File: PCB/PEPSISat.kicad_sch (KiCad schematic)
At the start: 3 parts, among them U1 STM32H747IITx, U2 RP2350A, U3 MT48LC16M16A2P

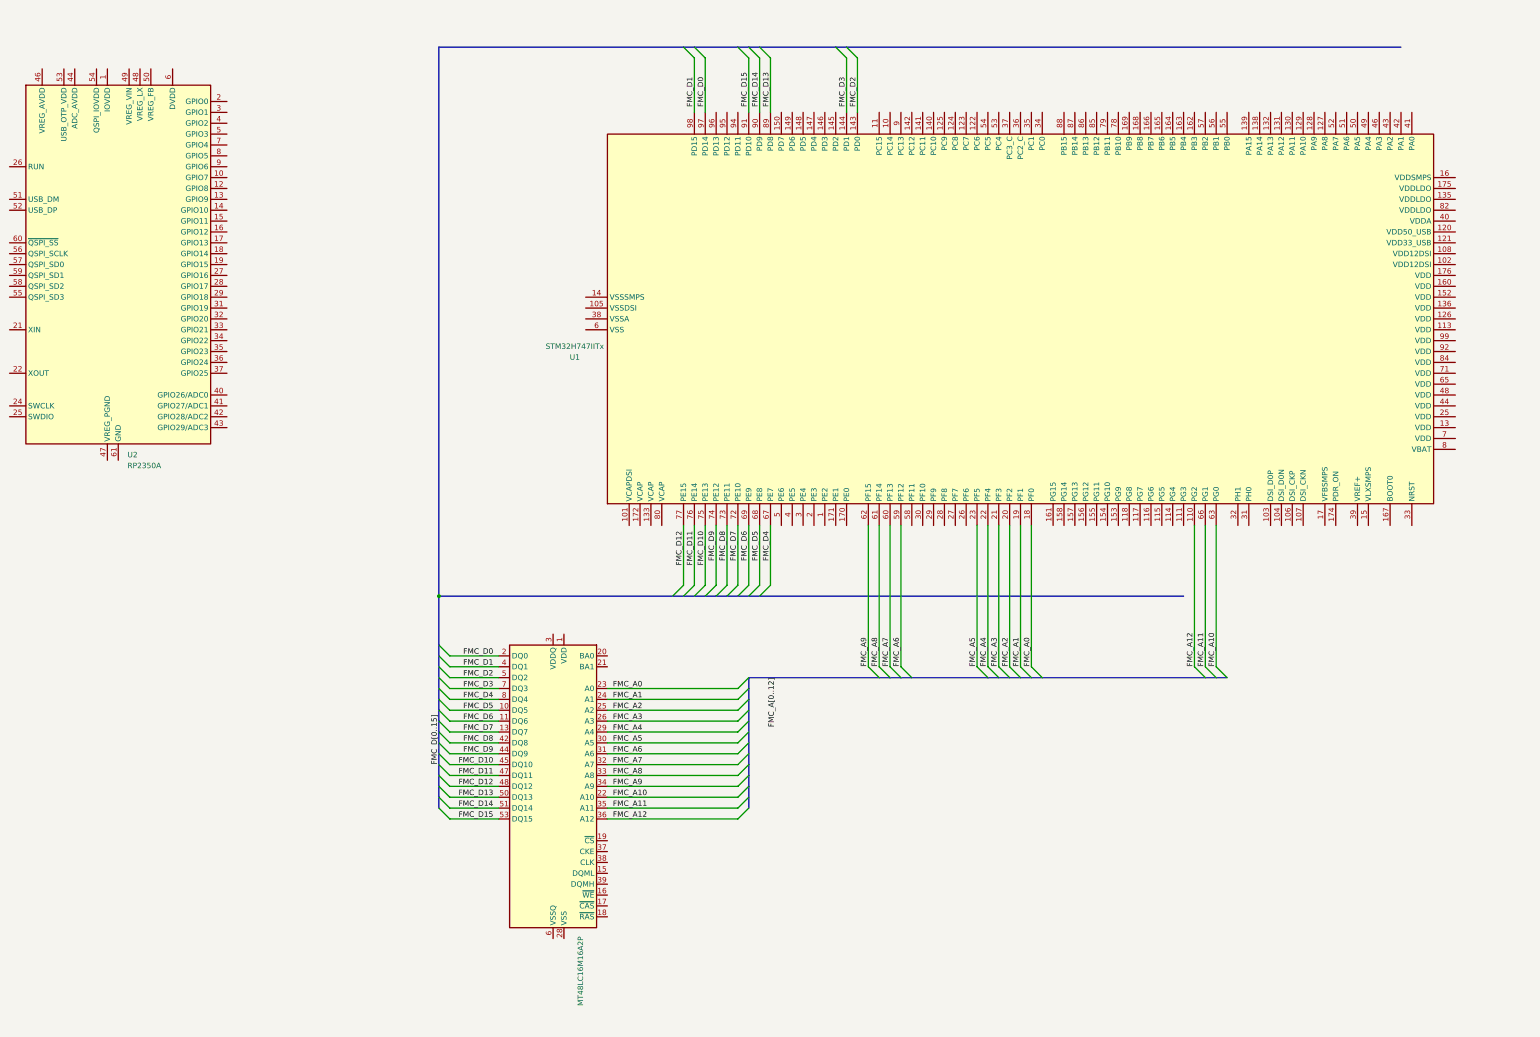
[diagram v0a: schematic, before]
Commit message: KiCad
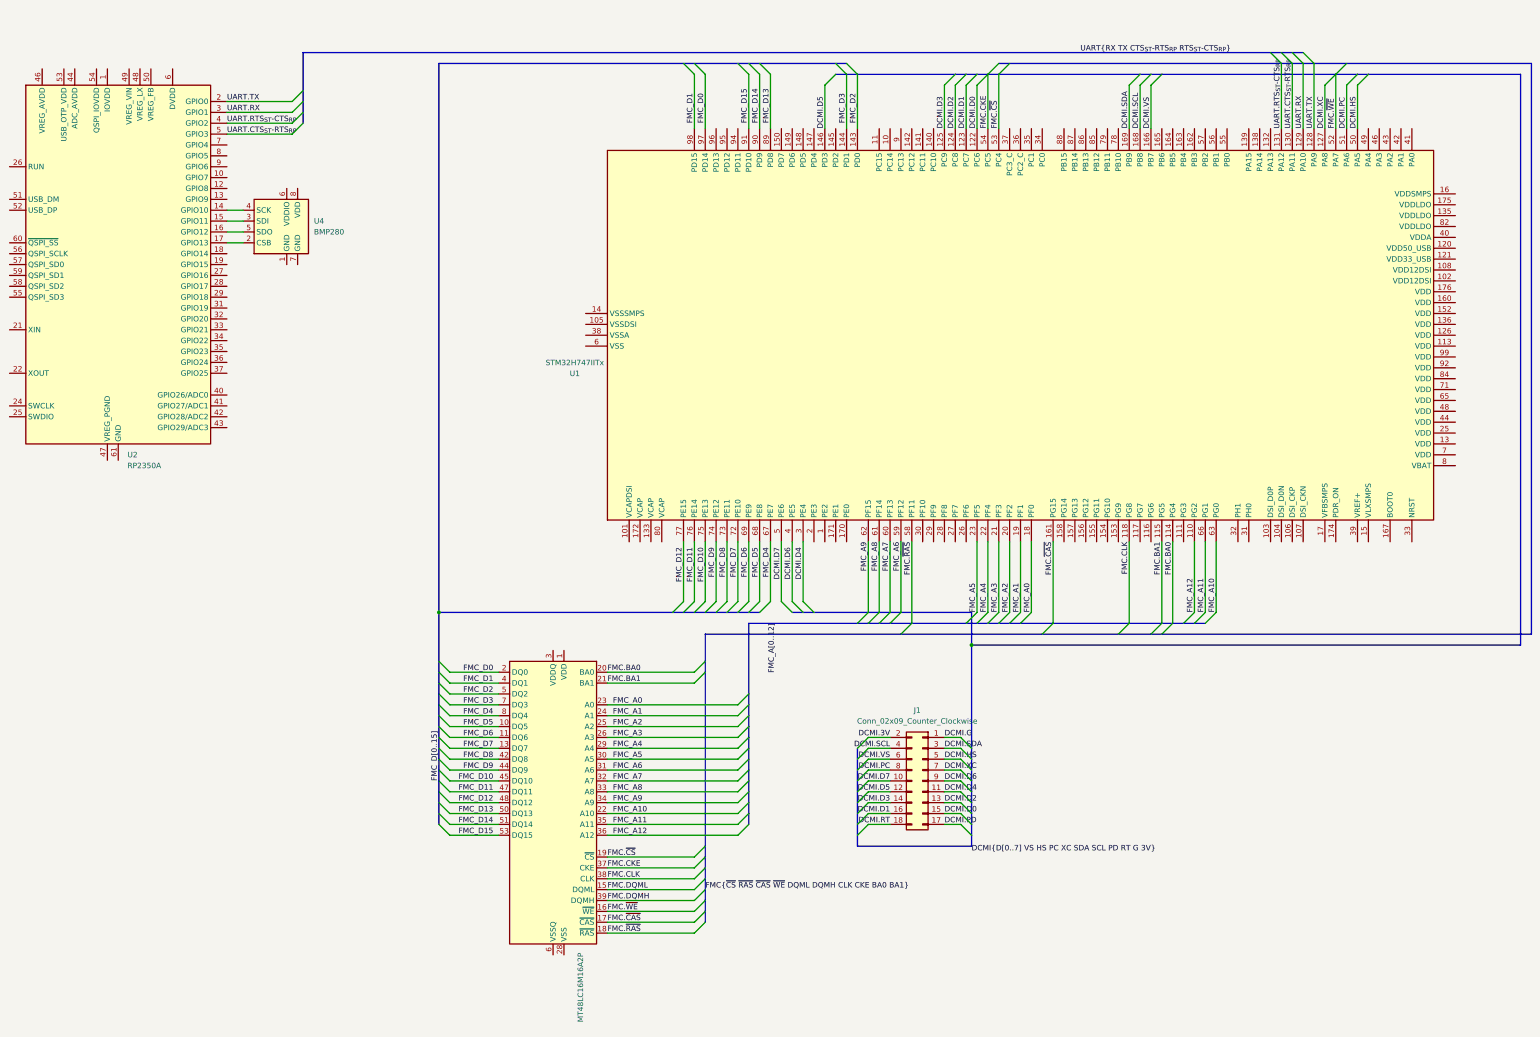
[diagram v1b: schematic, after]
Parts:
- added J1: Conn_02x09_Counter_Clockwise, Connector_PinHeader_2.54mm:PinHeader_2x09_P2.54mm_Horizontal, symbol Connector_Generic:Conn_02x09_Odd_Even
- added U4: BMP280, Package_LGA:Bosch_LGA-8_2x2.5mm_P0.65mm_ClockwisePinNumbering, symbol Sensor_Pressure:BMP280
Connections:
- net at U2.14 (GPIO10): now also U4.4 (SCK)
- net at U2.15 (GPIO11): now also U4.3 (SDI)
- net at U2.16 (GPIO12): now also U4.5 (SDO)
- net at U2.17 (GPIO13): now also U4.2 (CSB)
- net UART.TX: now reaches U2.2 (GPIO0)
- net UART.TX: now also U1.128 (PA9)
- net UART.RX: now reaches U2.3 (GPIO1)
- net UART.RX: now also U1.129 (PA10)
- net UART.RTS_{ST}-CTS_{RP}: now reaches U2.4 (GPIO2)
- net UART.RTS_{ST}-CTS_{RP}: now also U1.131 (PA12)
- net UART.CTS_{ST}-RTS_{RP}: now reaches U2.5 (GPIO3)
- net UART.CTS_{ST}-RTS_{RP}: now also U1.130 (PA11)
- net FMC.DQML: now reaches U3.15 (DQML)
- net FMC.~{WE}: now reaches U3.16 (~{WE})
- net FMC.~{WE}: now also U1.52 (PA7)
- net FMC.~{CAS}: now reaches U3.17 (~{CAS})
- net FMC.~{CAS}: now also U1.161 (PG15)
- net FMC.~{RAS}: now reaches U3.18 (~{RAS})
- net FMC.~{RAS}: now also U1.58 (PF11)
- net FMC.~{CS}: now reaches U3.19 (~{CS})
- net FMC.~{CS}: now also U1.53 (PC4)
- net FMC.BA0: now reaches U3.20 (BA0)
- net FMC.BA0: now also U1.114 (PG4)
- net FMC.BA1: now reaches U3.21 (BA1)
- net FMC.BA1: now also U1.115 (PG5)
- net FMC.CKE: now reaches U3.37 (CKE)
- net FMC.CKE: now also U1.54 (PC5)
- net FMC.CLK: now reaches U3.38 (CLK)
- net FMC.CLK: now also U1.118 (PG8)
- net FMC.DQMH: now reaches U3.39 (DQMH)
- net DCMI.D0: now reaches U1.122 (PC6)
- net DCMI.D0: now also J1.15 (Pin_15)
- net DCMI.D1: now reaches U1.123 (PC7)
- net DCMI.D1: now also J1.16 (Pin_16)
- net DCMI.D2: now reaches U1.124 (PC8)
- net DCMI.D2: now also J1.13 (Pin_13)
- net DCMI.D3: now reaches U1.125 (PC9)
- net DCMI.D3: now also J1.14 (Pin_14)
- net DCMI.XC: now reaches U1.127 (PA8)
- net DCMI.XC: now also J1.7 (Pin_7)
- net DCMI.D5: now reaches U1.146 (PD3)
- net DCMI.D5: now also J1.12 (Pin_12)
- net DCMI.VS: now reaches U1.166 (PB7)
- net DCMI.VS: now also J1.6 (Pin_6)
- net DCMI.SCL: now reaches U1.168 (PB8)
- net DCMI.SCL: now also J1.4 (Pin_4)
- net DCMI.SDA: now reaches U1.169 (PB9)
- net DCMI.SDA: now also J1.3 (Pin_3)
- net DCMI.D4: now reaches U1.3 (PE4)
- net DCMI.D4: now also J1.11 (Pin_11)
- net DCMI.D6: now reaches U1.4 (PE5)
- net DCMI.D6: now also J1.9 (Pin_9)
- net DCMI.D7: now reaches U1.5 (PE6)
- net DCMI.D7: now also J1.10 (Pin_10)
- net DCMI.HS: now reaches U1.50 (PA5)
- net DCMI.HS: now also J1.5 (Pin_5)
- net DCMI.PC: now reaches U1.51 (PA6)
- net DCMI.PC: now also J1.8 (Pin_8)
- new net DCMI.3V: J1.2 (Pin_2)
- new net DCMI.G: J1.1 (Pin_1)
- new net DCMI.PD: J1.17 (Pin_17)
- new net DCMI.RT: J1.18 (Pin_18)
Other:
- moved on the sheet: U1

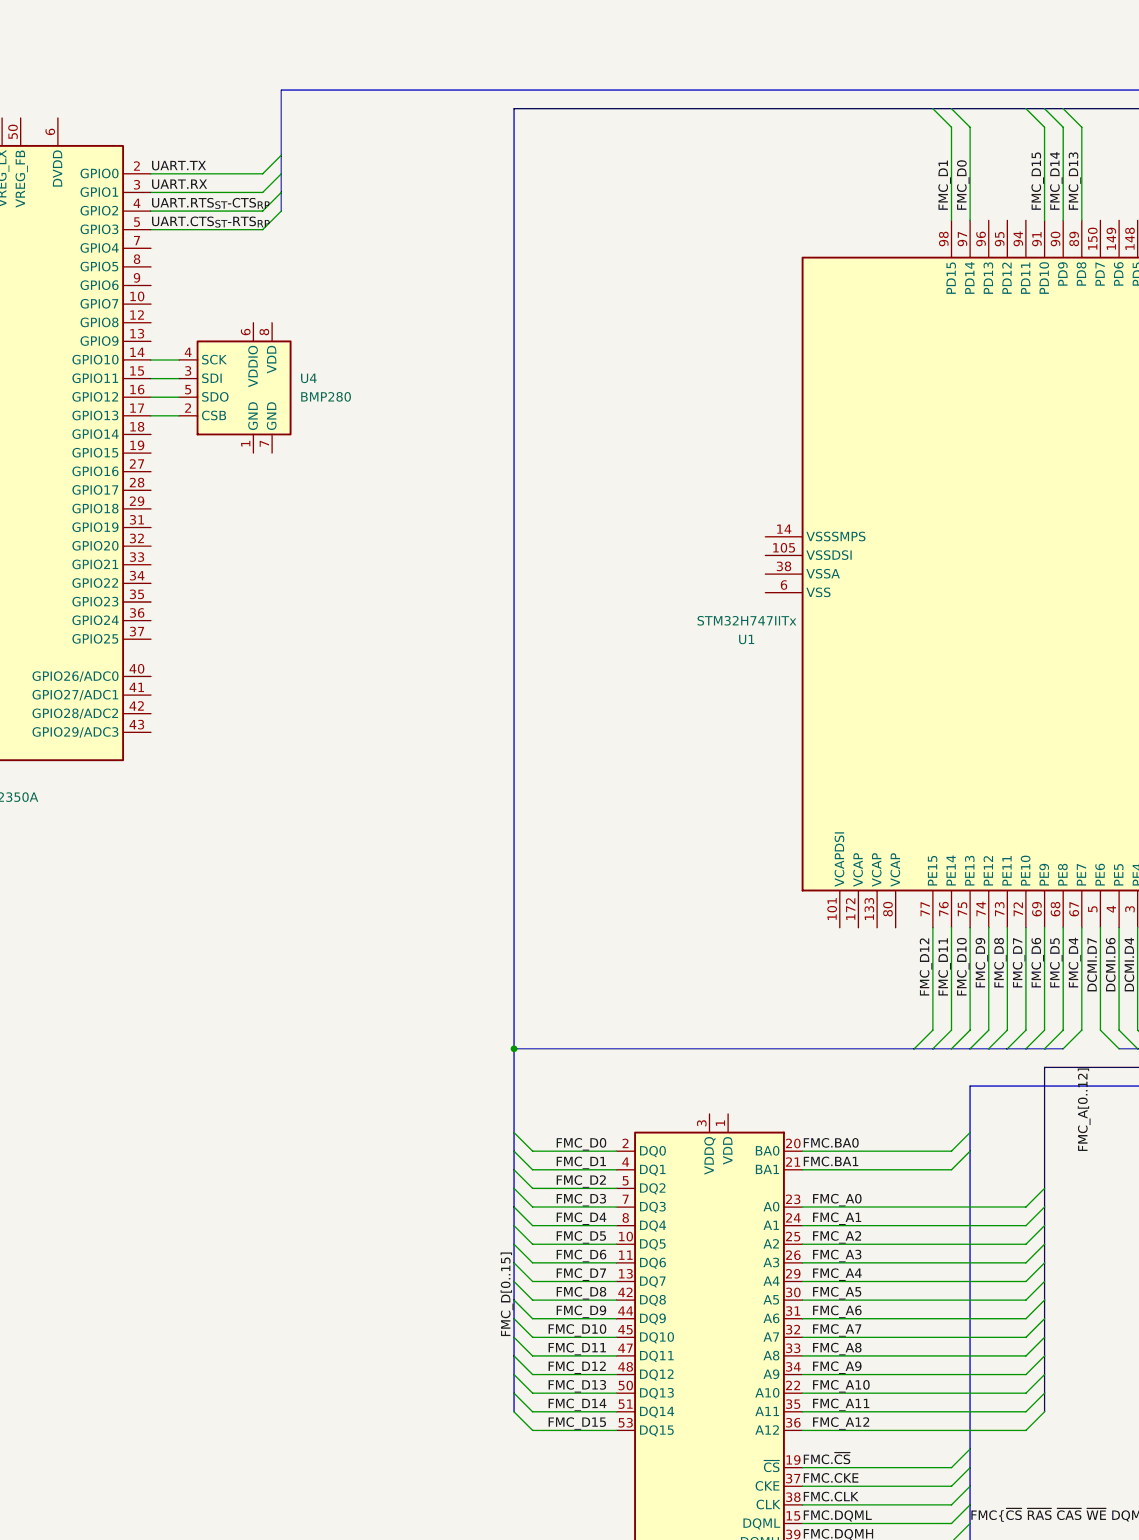
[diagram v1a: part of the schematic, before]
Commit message: KiCad
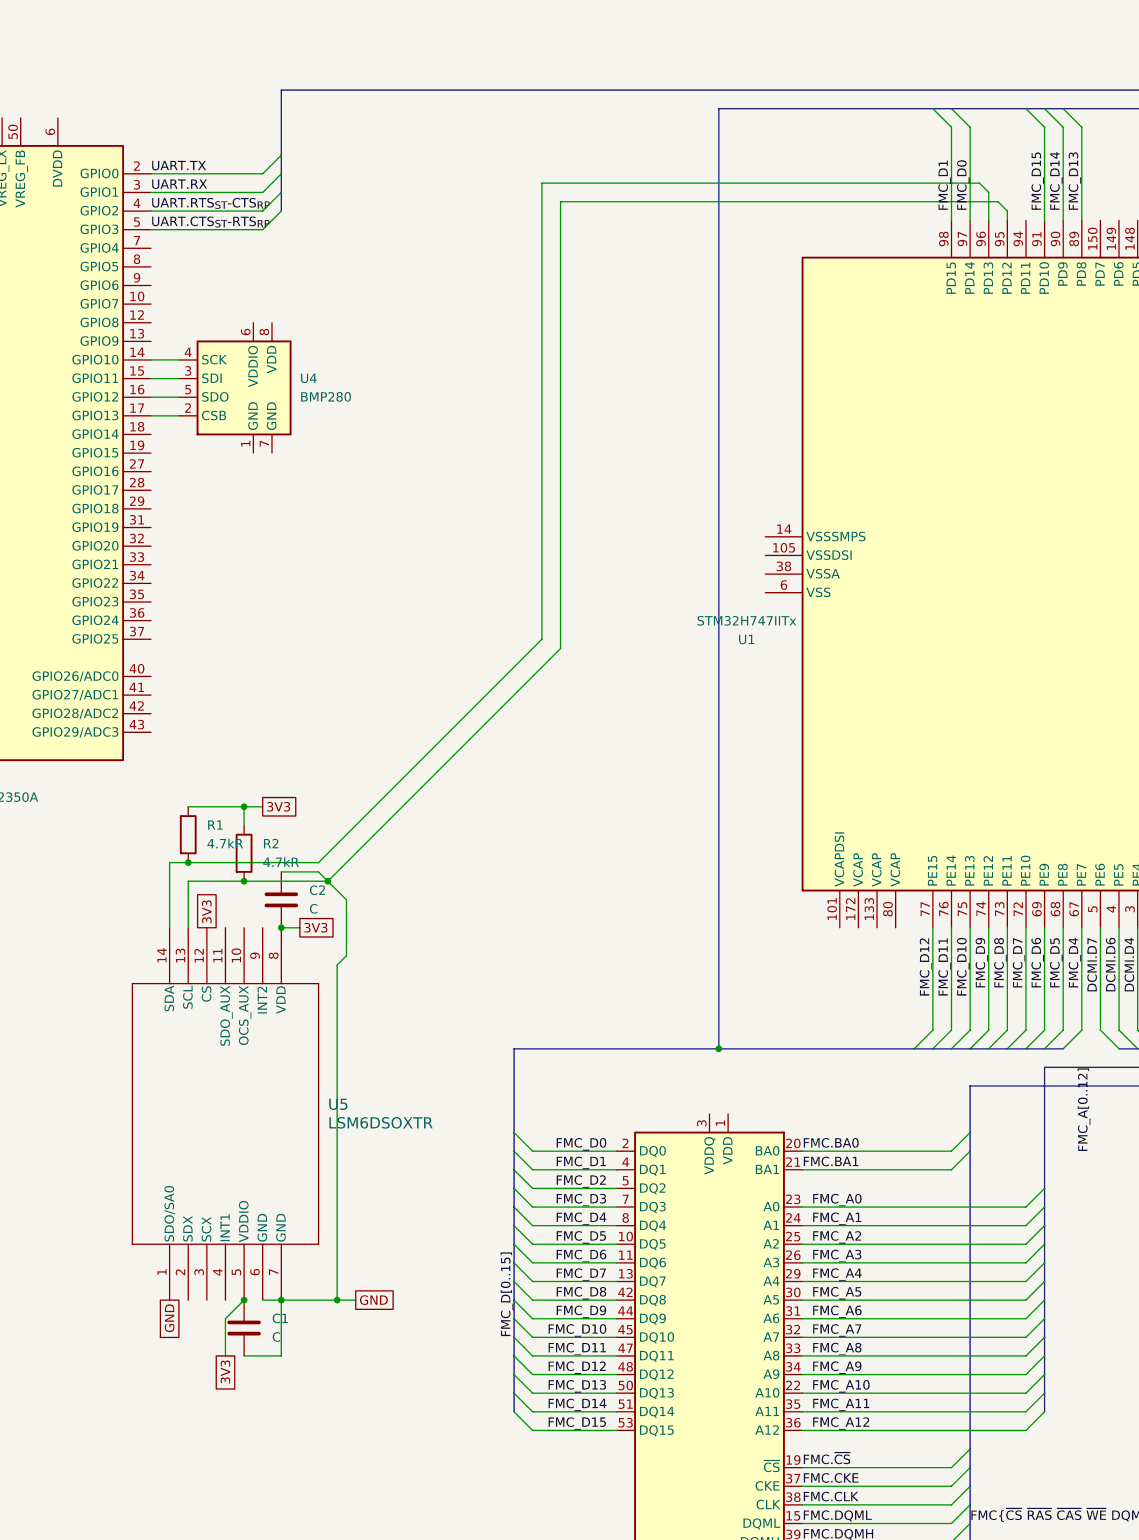
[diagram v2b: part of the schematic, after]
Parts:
- added C1, C2: C, symbol Device:C
- added R1, R2: 4.7kR, Resistor_SMD:R_0603_1608Metric, symbol Device:R
- added U5: LSM6DSOXTR, LGA-14L_STM, symbol LSM6DSOXTR:LSM6DSOXTR
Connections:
- net GND: now reaches U1.95 (PD12)
- net GND: now also C1.2, C2.1, R2.2, U5.1 (SDO/SA0), U5.13 (SCL), U5.6 (GND), U5.7 (GND)
- net at U1.96 (PD13): now also R1.2, U5.14 (SDA)
- new net 3V3: C1.1, C2.2, R1.1, R2.1, U5.12 (CS), U5.5 (VDDIO), U5.8 (VDD)
